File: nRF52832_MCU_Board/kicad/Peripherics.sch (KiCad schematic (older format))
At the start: 17 parts, among them J1 CONN_01X03, J2 CONN_01X16, J3 CONN_01X08, J4 CONN_01X03, J9 CONN_01X08

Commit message: Update KiCad project nRF52832_MCU_Board
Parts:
- J2: footprint Pin_Headers:Pin_Header_Straight_1x16_Pitch2.54mm -> Nordic_misc:Pin_Header_Straight_1x16_Pitch2.54mm
- J3, J9: footprint Pin_Headers:Pin_Header_Straight_1x08_Pitch2.54mm -> Nordic_misc:Pin_Header_Straight_1x08_Pitch2.54mm
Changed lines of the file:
@@
 F 0 "J2" H 10000 2800 50  0000 C CNN
 F 1 "CONN_01X16" V 10100 1950 50  0000 C CNN
-F 2 "Pin_Headers:Pin_Header_Straight_1x16_Pitch2.54mm" H 10000 1950 50  0001 C CNN
+F 2 "Nordic_misc:Pin_Header_Straight_1x16_Pitch2.54mm" H 10000 1950 50  0001 C CNN
 F 3 "" H 10000 1950 50  0001 C CNN
 	1    10000 1950
@@
 F 0 "J3" H 4900 1950 50  0000 C CNN
 F 1 "CONN_01X08" V 5000 1500 50  0000 C CNN
-F 2 "Pin_Headers:Pin_Header_Straight_1x08_Pitch2.54mm" H 4900 1500 50  0001 C CNN
+F 2 "Nordic_misc:Pin_Header_Straight_1x08_Pitch2.54mm" H 4900 1500 50  0001 C CNN
 F 3 "" H 4900 1500 50  0001 C CNN
 	1    4900 1500
@@
 F 0 "J9" H 4900 3000 50  0000 C CNN
 F 1 "CONN_01X08" V 5000 2550 50  0000 C CNN
-F 2 "Pin_Headers:Pin_Header_Straight_1x08_Pitch2.54mm" H 4900 2550 50  0001 C CNN
+F 2 "Nordic_misc:Pin_Header_Straight_1x08_Pitch2.54mm" H 4900 2550 50  0001 C CNN
 F 3 "" H 4900 2550 50  0001 C CNN
 	1    4900 2550

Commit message: Update KiCad Project nRF52832_MCU_Board
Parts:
- J1, J4: footprint Pin_Headers:Pin_Header_Straight_1x03_Pitch2.54mm_SMD_Pin1Left -> Nordic_misc:bb02-hy03a
- J2: footprint Nordic_misc:Pin_Header_Straight_1x16_Pitch2.54mm -> Nordic_misc:bb02-hy16a
- J3, J9: footprint Nordic_misc:Pin_Header_Straight_1x08_Pitch2.54mm -> Nordic_misc:bb02-hy08a
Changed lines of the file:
@@
 F 0 "J2" H 10000 2800 50  0000 C CNN
 F 1 "CONN_01X16" V 10100 1950 50  0000 C CNN
-F 2 "Nordic_misc:Pin_Header_Straight_1x16_Pitch2.54mm" H 10000 1950 50  0001 C CNN
+F 2 "Nordic_misc:bb02-hy16a" H 10000 1950 50  0001 C CNN
 F 3 "" H 10000 1950 50  0001 C CNN
 	1    10000 1950
@@
 F 0 "J4" H 6400 1800 50  0000 C CNN
 F 1 "CONN_01X03" V 6500 1600 50  0000 C CNN
-F 2 "Pin_Headers:Pin_Header_Straight_1x03_Pitch2.54mm_SMD_Pin1Left" H 6400 1600 50  0001 C CNN
+F 2 "Nordic_misc:bb02-hy03a" H 6400 1600 50  0001 C CNN
 F 3 "" H 6400 1600 50  0001 C CNN
 	1    6400 1600
@@
 F 0 "J1" H 8550 1800 50  0000 C CNN
 F 1 "CONN_01X03" V 8650 1600 50  0000 C CNN
-F 2 "Pin_Headers:Pin_Header_Straight_1x03_Pitch2.54mm_SMD_Pin1Left" H 8550 1600 50  0001 C CNN
+F 2 "Nordic_misc:bb02-hy03a" H 8550 1600 50  0001 C CNN
 F 3 "" H 8550 1600 50  0001 C CNN
 	1    8550 1600
@@
 F 0 "J3" H 4900 1950 50  0000 C CNN
 F 1 "CONN_01X08" V 5000 1500 50  0000 C CNN
-F 2 "Nordic_misc:Pin_Header_Straight_1x08_Pitch2.54mm" H 4900 1500 50  0001 C CNN
+F 2 "Nordic_misc:bb02-hy08a" H 4900 1500 50  0001 C CNN
 F 3 "" H 4900 1500 50  0001 C CNN
 	1    4900 1500
@@
 F 0 "J9" H 4900 3000 50  0000 C CNN
 F 1 "CONN_01X08" V 5000 2550 50  0000 C CNN
-F 2 "Nordic_misc:Pin_Header_Straight_1x08_Pitch2.54mm" H 4900 2550 50  0001 C CNN
+F 2 "Nordic_misc:bb02-hy08a" H 4900 2550 50  0001 C CNN
 F 3 "" H 4900 2550 50  0001 C CNN
 	1    4900 2550

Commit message: Update KiCAD Project nRF52832_MCU_Board
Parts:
- D1, D2, D3: footprint LEDs:LED_0603 -> Nordic_misc:LED_0603
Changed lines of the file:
@@
 F 0 "D2" H 5600 4600 50  0000 C CNN
 F 1 "LED" H 5600 4400 50  0000 C CNN
-F 2 "LEDs:LED_0603" H 5600 4500 50  0001 C CNN
+F 2 "Nordic_misc:LED_0603" H 5600 4500 50  0001 C CNN
 F 3 "" H 5600 4500 50  0001 C CNN
 	1    5600 4500
@@
 F 0 "D3" H 5950 4600 50  0000 C CNN
 F 1 "LED" H 5950 4400 50  0000 C CNN
-F 2 "LEDs:LED_0603" H 5950 4500 50  0001 C CNN
+F 2 "Nordic_misc:LED_0603" H 5950 4500 50  0001 C CNN
 F 3 "" H 5950 4500 50  0001 C CNN
 	1    5950 4500
@@
 F 0 "D1" H 6350 4600 50  0000 C CNN
 F 1 "LED" H 6350 4400 50  0000 C CNN
-F 2 "LEDs:LED_0603" H 6350 4500 50  0001 C CNN
+F 2 "Nordic_misc:LED_0603" H 6350 4500 50  0001 C CNN
 F 3 "" H 6350 4500 50  0001 C CNN
 	1    6350 4500

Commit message: Update KiCAD Project nRF52832_MCU_Board
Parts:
- J1, J4: footprint Nordic_misc:bb02-hy03a -> Nordic_misc:Pin_Header_Straight_1x03_Pitch2.54mm
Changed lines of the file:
@@
 EESchema Schematic File Version 2
-LIBS:power
-LIBS:device
-LIBS:transistors
-LIBS:conn
-LIBS:linear
-LIBS:regul
+LIBS:nRF52832_MCU_Board-rescue
+LIBS:Nordic_misc
+LIBS:Nordic_nRF
+LIBS:74xgxx
 LIBS:74xx
-LIBS:cmos4000
-LIBS:adc-dac
-LIBS:memory
-LIBS:xilinx
-LIBS:microcontrollers
-LIBS:dsp
-LIBS:microchip
-LIBS:analog_switches
-LIBS:motorola
-LIBS:texas
-LIBS:intel
-LIBS:audio
-LIBS:interface
-LIBS:digital-audio
-LIBS:philips
-LIBS:display
-LIBS:cypress
-LIBS:siliconi
-LIBS:opto
-LIBS:atmel
-LIBS:contrib
-LIBS:valves
-LIBS:74xgxx
 LIBS:ac-dc
 LIBS:actel
+LIBS:adc-dac
 LIBS:allegro
 LIBS:Altera
 LIBS:analog_devices
+LIBS:analog_switches
+LIBS:atmel
+LIBS:audio
 LIBS:battery_management
 LIBS:bbd
@@
 LIBS:brooktre
 LIBS:cmos_ieee
+LIBS:cmos4000
+LIBS:conn
+LIBS:contrib
+LIBS:cypress
 LIBS:dc-dc
+LIBS:device
+LIBS:digital-audio
 LIBS:diode
+LIBS:display
+LIBS:dsp
 LIBS:elec-unifil
 LIBS:ESD_Protection
@@
 LIBS:graphic
 LIBS:hc11
+LIBS:intel
+LIBS:interface
 LIBS:ir
 LIBS:Lattice
 LIBS:leds
+LIBS:linear
 LIBS:logo
 LIBS:maxim
 LIBS:mechanical
+LIBS:memory
+LIBS:microchip
 LIBS:microchip_dspic33dsc
 LIBS:microchip_pic10mcu
@@
 LIBS:microchip_pic24mcu
 LIBS:microchip_pic32mcu
+LIBS:microcontrollers
 LIBS:modules
 LIBS:motor_drivers
+LIBS:motorola
 LIBS:motors
 LIBS:msp430
@@
 LIBS:nxp_armmcu
 LIBS:onsemi
-LIBS:OPA4134
+LIBS:opto
 LIBS:Oscillators
-LIBS:PCM3168A
+LIBS:philips
+LIBS:power
+LIBS:Power_Management
 LIBS:powerint
-LIBS:Power_Management
 LIBS:pspice
 LIBS:references
+LIBS:regul
 LIBS:relays
 LIBS:rfcom
 LIBS:sensors
 LIBS:silabs
+LIBS:siliconi
 LIBS:stm8
 LIBS:stm32
 LIBS:supertex
 LIBS:switches
-LIBS:TMS320VC5502
+LIBS:texas
 LIBS:transf
+LIBS:transistors
 LIBS:triac_thyristor
-LIBS:TS3A27518E
 LIBS:ttl_ieee
+LIBS:valves
 LIBS:video
 LIBS:w_analog
-LIBS:w_connectors
 LIBS:w_device
-LIBS:wiznet
 LIBS:w_logic
 LIBS:w_memory
 LIBS:w_microcontrollers
 LIBS:w_opto
-LIBS:Worldsemi
 LIBS:w_relay
 LIBS:w_rtx
 LIBS:w_transistor
 LIBS:w_vacuum
+LIBS:wiznet
+LIBS:Worldsemi
 LIBS:Xicor
+LIBS:xilinx
 LIBS:zetex
 LIBS:Zilog
-LIBS:Nordic_misc
-LIBS:Nordic_nRF
 LIBS:nRF52832_MCU_Board-cache
 EELAYER 25 0
@@
 U 1 1 597D6C73
 P 5600 4500
+AR Path="/597D6C73" Ref="D2"  Part="1"
+AR Path="/597D3B45/597D6C73" Ref="D2"  Part="1"
 F 0 "D2" H 5600 4600 50  0000 C CNN
 F 1 "LED" H 5600 4400 50  0000 C CNN
@@
 U 1 1 597D6D22
 P 5950 4500
+AR Path="/597D6D22" Ref="D3"  Part="1"
+AR Path="/597D3B45/597D6D22" Ref="D3"  Part="1"
 F 0 "D3" H 5950 4600 50  0000 C CNN
 F 1 "LED" H 5950 4400 50  0000 C CNN
@@
 U 1 1 597D6D42
 P 6350 4500
+AR Path="/597D6D42" Ref="D1"  Part="1"
+AR Path="/597D3B45/597D6D42" Ref="D1"  Part="1"
 F 0 "D1" H 6350 4600 50  0000 C CNN
 F 1 "LED" H 6350 4400 50  0000 C CNN
@@
 F 0 "J4" H 6400 1800 50  0000 C CNN
 F 1 "CONN_01X03" V 6500 1600 50  0000 C CNN
-F 2 "Nordic_misc:bb02-hy03a" H 6400 1600 50  0001 C CNN
+F 2 "Nordic_misc:Pin_Header_Straight_1x03_Pitch2.54mm" H 6400 1600 50  0001 C CNN
 F 3 "" H 6400 1600 50  0001 C CNN
 	1    6400 1600
@@
 F 0 "J1" H 8550 1800 50  0000 C CNN
 F 1 "CONN_01X03" V 8650 1600 50  0000 C CNN
-F 2 "Nordic_misc:bb02-hy03a" H 8550 1600 50  0001 C CNN
+F 2 "Nordic_misc:Pin_Header_Straight_1x03_Pitch2.54mm" H 8550 1600 50  0001 C CNN
 F 3 "" H 8550 1600 50  0001 C CNN
 	1    8550 1600

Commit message: Update KiCAD Project nRF52832_MCU_Board
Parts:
- BTN1, BTN2: footprint Buttons_Switches_SMD:SW_SPST_PTS645 -> Nordic_misc:Nordic_misc-PANASONIC_EVQPT5A15
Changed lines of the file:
@@
 F 0 "BTN1" H 8650 5120 45  0000 L BNN
 F 1 "PANASONIC_EVQPT5A15" H 8950 4550 39  0000 C CNN
-F 2 "Buttons_Switches_SMD:SW_SPST_PTS645" H 8680 4750 20  0001 C CNN
+F 2 "Nordic_misc:Nordic_misc-PANASONIC_EVQPT5A15" H 8680 4750 20  0001 C CNN
 F 3 "" H 8650 4600 60  0001 C CNN
 	1    8650 4600
@@
 F 0 "BTN2" H 8650 6270 45  0000 L BNN
 F 1 "PANASONIC_EVQPT5A15" H 8950 5700 39  0000 C CNN
-F 2 "Buttons_Switches_SMD:SW_SPST_PTS645" H 8680 5900 20  0001 C CNN
+F 2 "Nordic_misc:Nordic_misc-PANASONIC_EVQPT5A15" H 8680 5900 20  0001 C CNN
 F 3 "" H 8650 5750 60  0001 C CNN
 	1    8650 5750

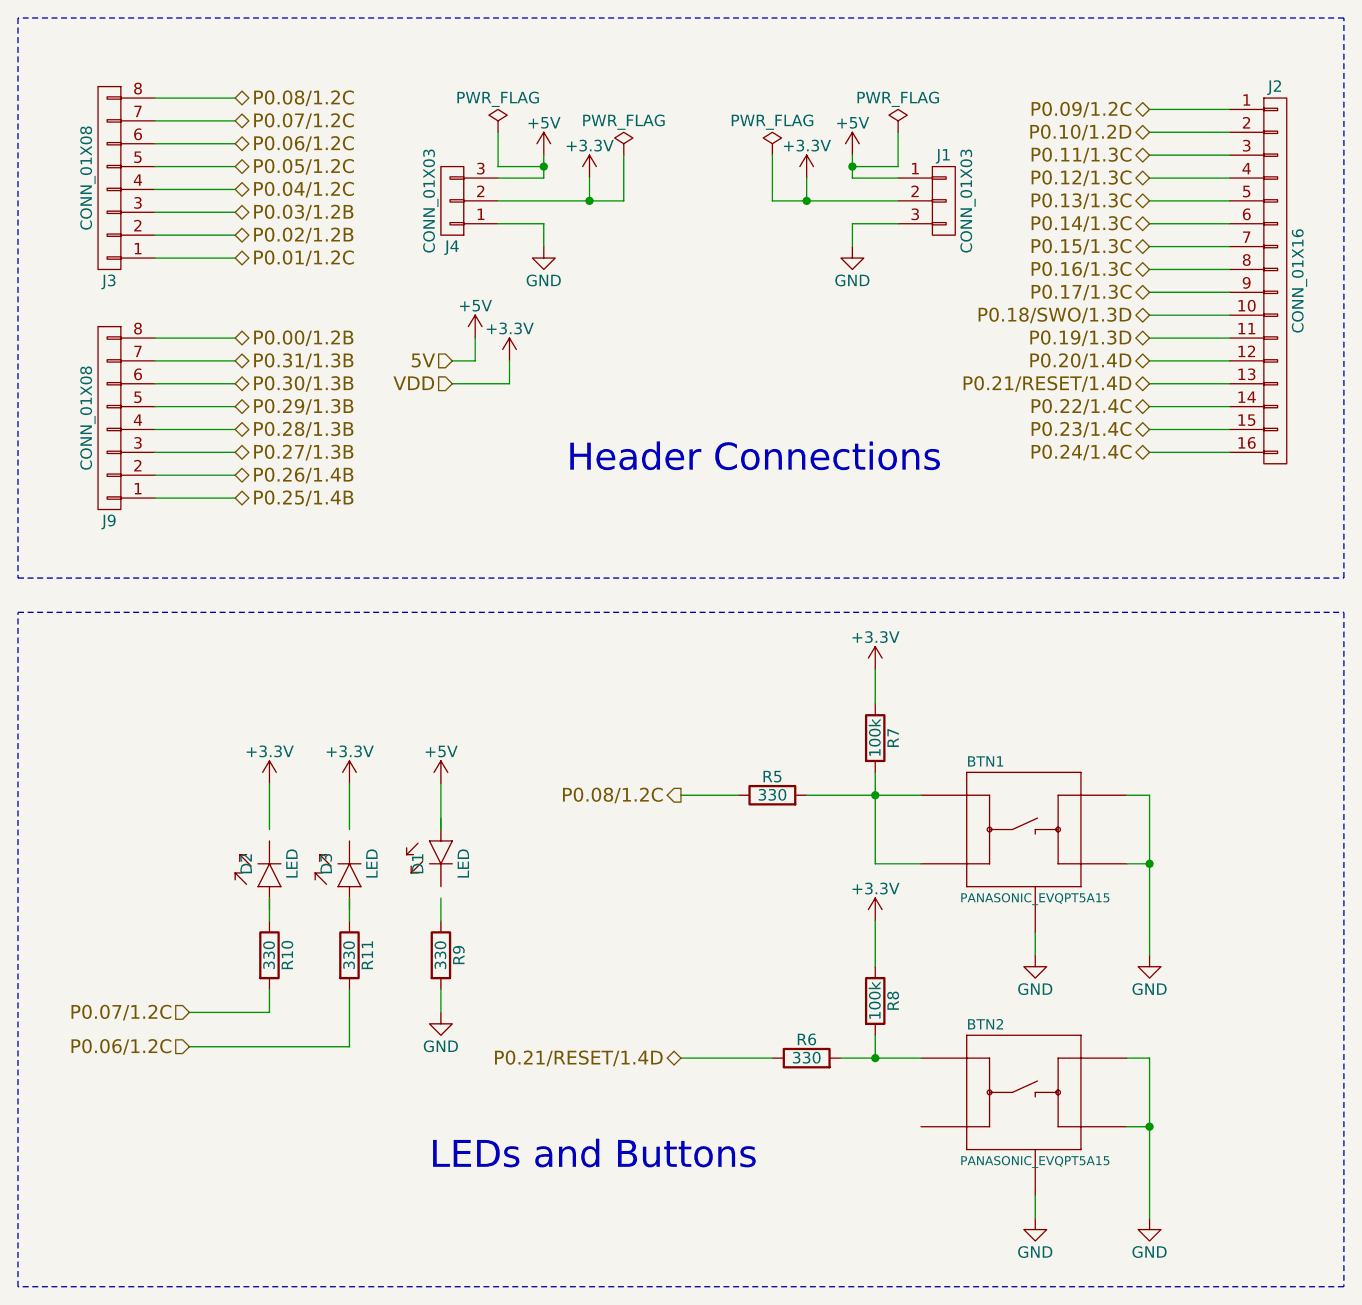
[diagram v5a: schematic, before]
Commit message: Update  KiCAD Project nRF52832_MCU_Board
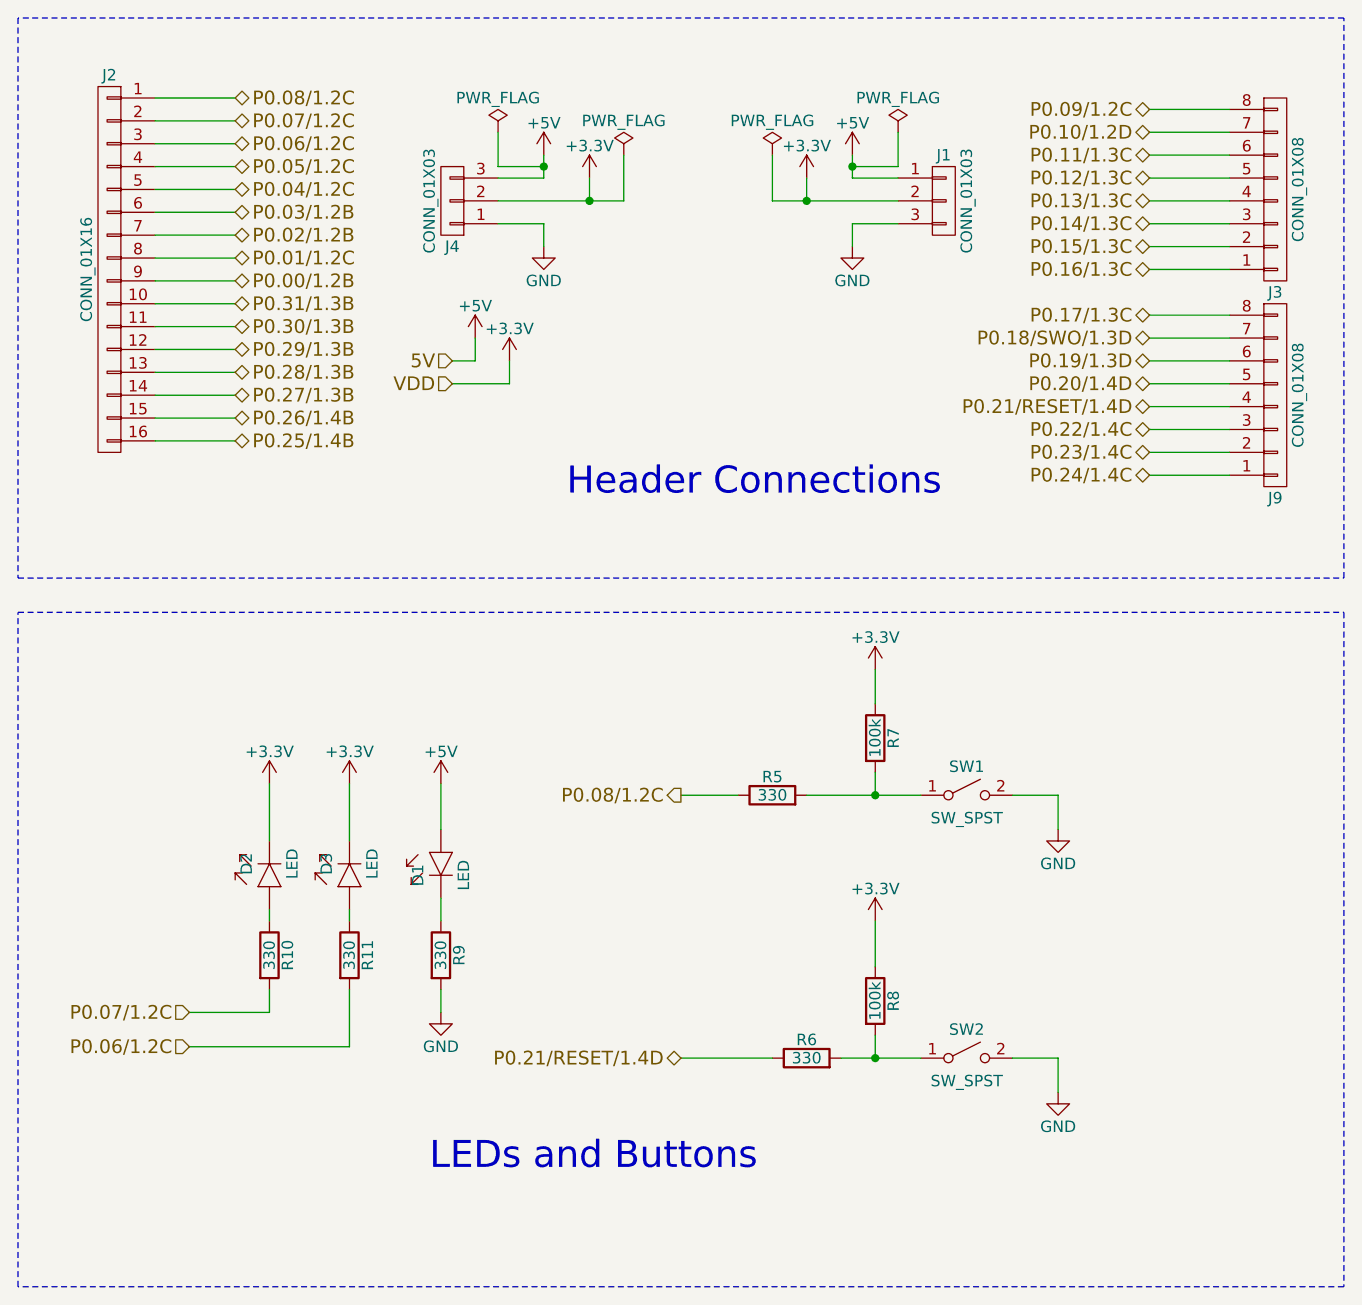
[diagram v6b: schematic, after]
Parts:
- removed BTN1, BTN2: PANASONIC_EVQPT5A15, Nordic_misc:Nordic_misc-PANASONIC_EVQPT5A15, symbol PANASONIC_EVQPT5A15
- added SW1, SW2: SW_SPST, Nordic_misc:SW_SPST_FSMSM, symbol SW_SPST
- J2: footprint Nordic_misc:bb02-hy16a -> Nordic_misc:Pin_Header_Straight_1x16_Pitch2.54mm
- J3, J9: footprint Nordic_misc:bb02-hy08a -> Nordic_misc:Pin_Header_Straight_1x08_Pitch2.54mm
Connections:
- wire segments 82 -> 77
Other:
- moved on the sheet: D1, J2, J3, J9
